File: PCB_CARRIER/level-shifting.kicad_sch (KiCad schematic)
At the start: 2 parts, among them U1 SN74LVC8T245, U2 SN74LVC2T45DCUR

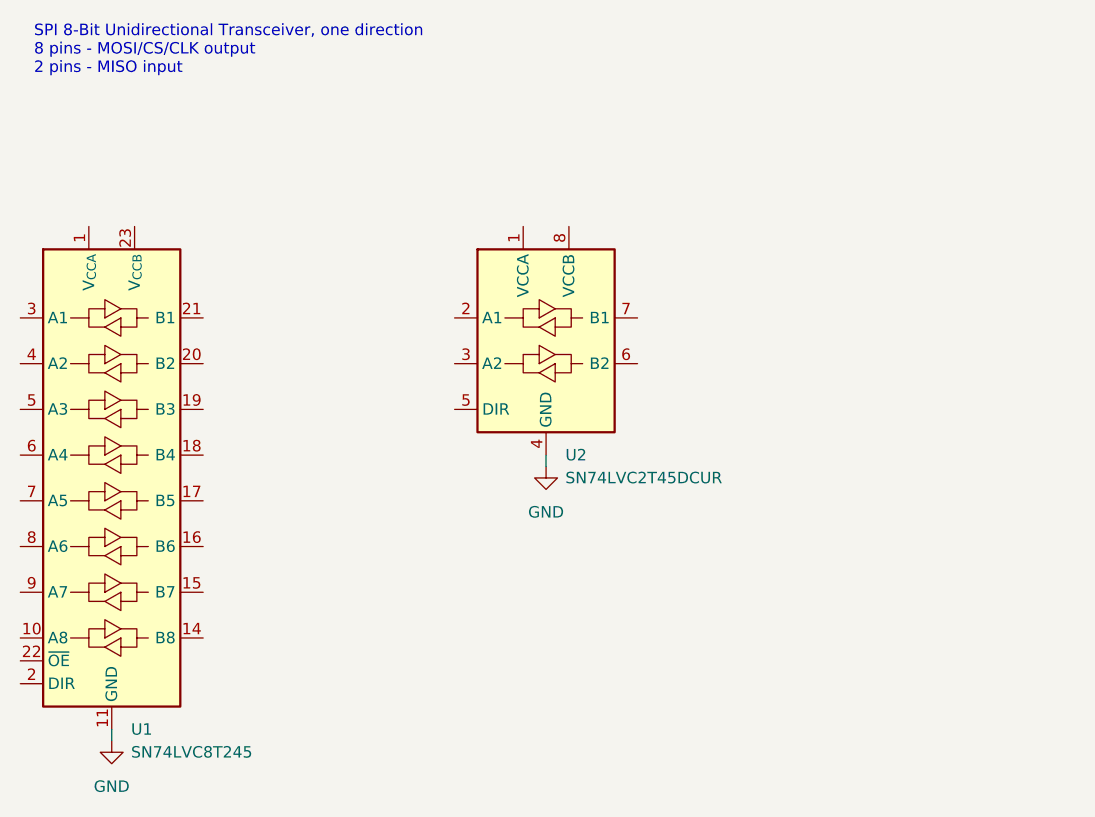
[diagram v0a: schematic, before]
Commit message: SPI inputs to level shift
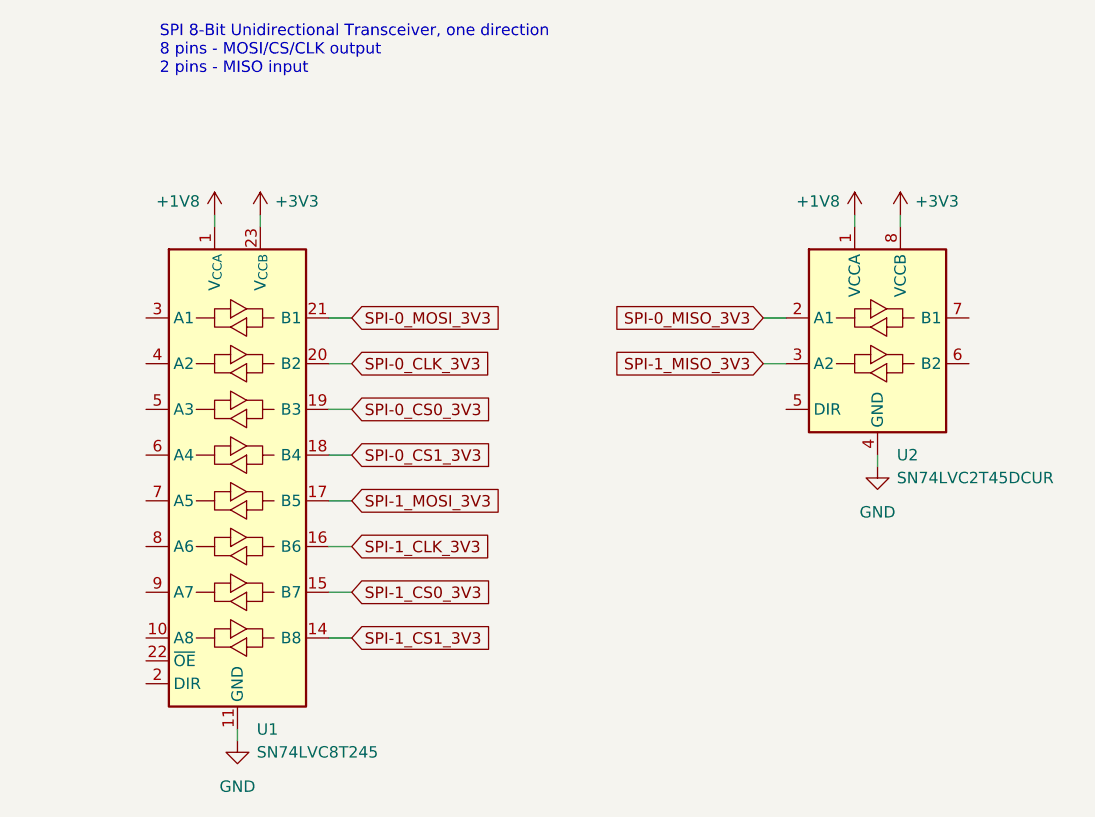
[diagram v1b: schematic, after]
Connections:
- net +1V8: now reaches U1.1 (V_{CCA})
- net +1V8: now also U2.1 (VCCA)
- net SPI-1_CS1_3V3: now reaches U1.14 (B8)
- net SPI-1_CS0_3V3: now reaches U1.15 (B7)
- net SPI-1_CLK_3V3: now reaches U1.16 (B6)
- net SPI-1_MOSI_3V3: now reaches U1.17 (B5)
- net SPI-0_CS1_3V3: now reaches U1.18 (B4)
- net SPI-0_CS0_3V3: now reaches U1.19 (B3)
- net SPI-0_CLK_3V3: now reaches U1.20 (B2)
- net SPI-0_MOSI_3V3: now reaches U1.21 (B1)
- net +3V3: now reaches U1.23 (V_{CCB}), U1.24 (V_{CCB})
- net +3V3: now also U2.8 (VCCB)
- net SPI-0_MISO_3V3: now reaches U2.2 (A1)
- net SPI-1_MISO_3V3: now reaches U2.3 (A2)
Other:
- moved on the sheet: U1, U2
